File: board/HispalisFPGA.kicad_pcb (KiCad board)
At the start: 4 copper layers, 91.3 x 79.9 mm, 133 parts, among them J1 HC-TYPE-C-16P-01A, Q1 DMG1012T, Q2 DMG1012T, Q3 DMG1012T, Q4 DMG1012T, SW1 SW_DIP_x08, U1 93LC46B, U2 FT2232HQ, Y1 12MHz

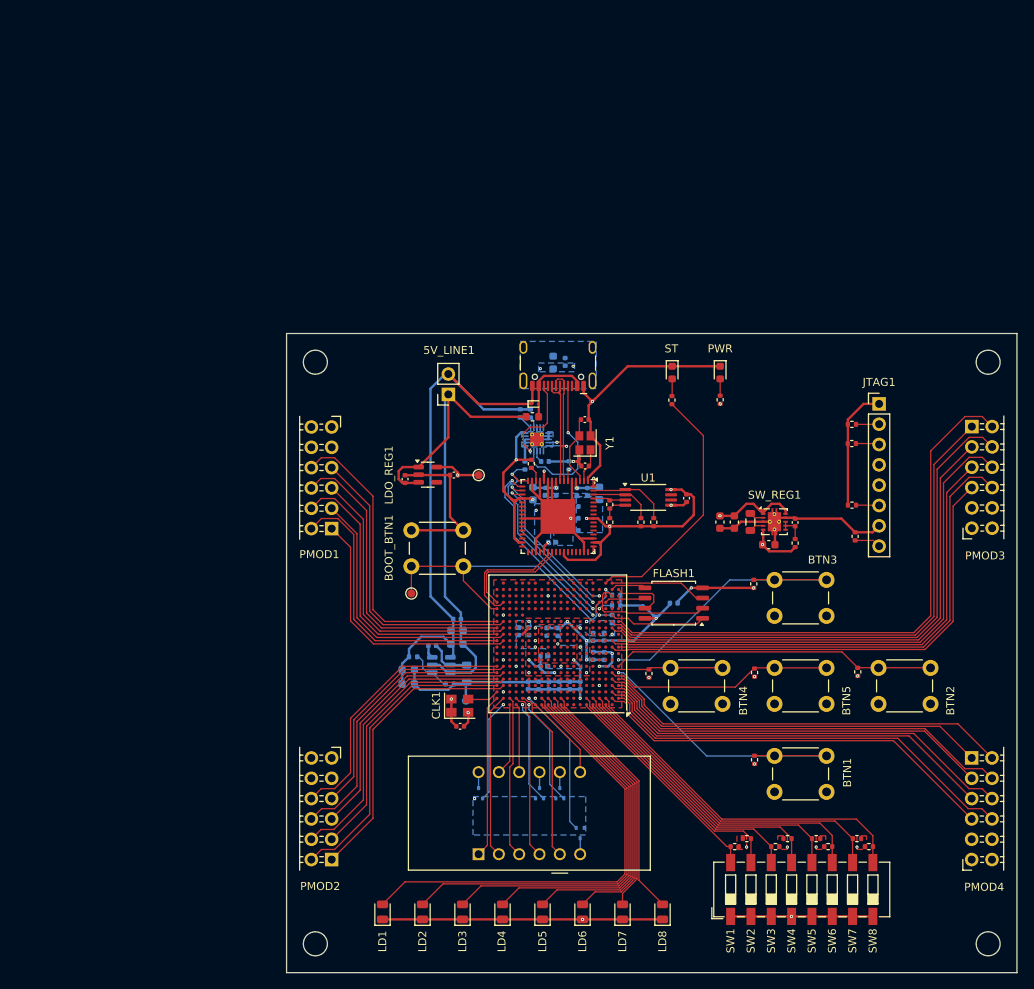
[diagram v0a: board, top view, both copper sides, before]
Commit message: Add metadata
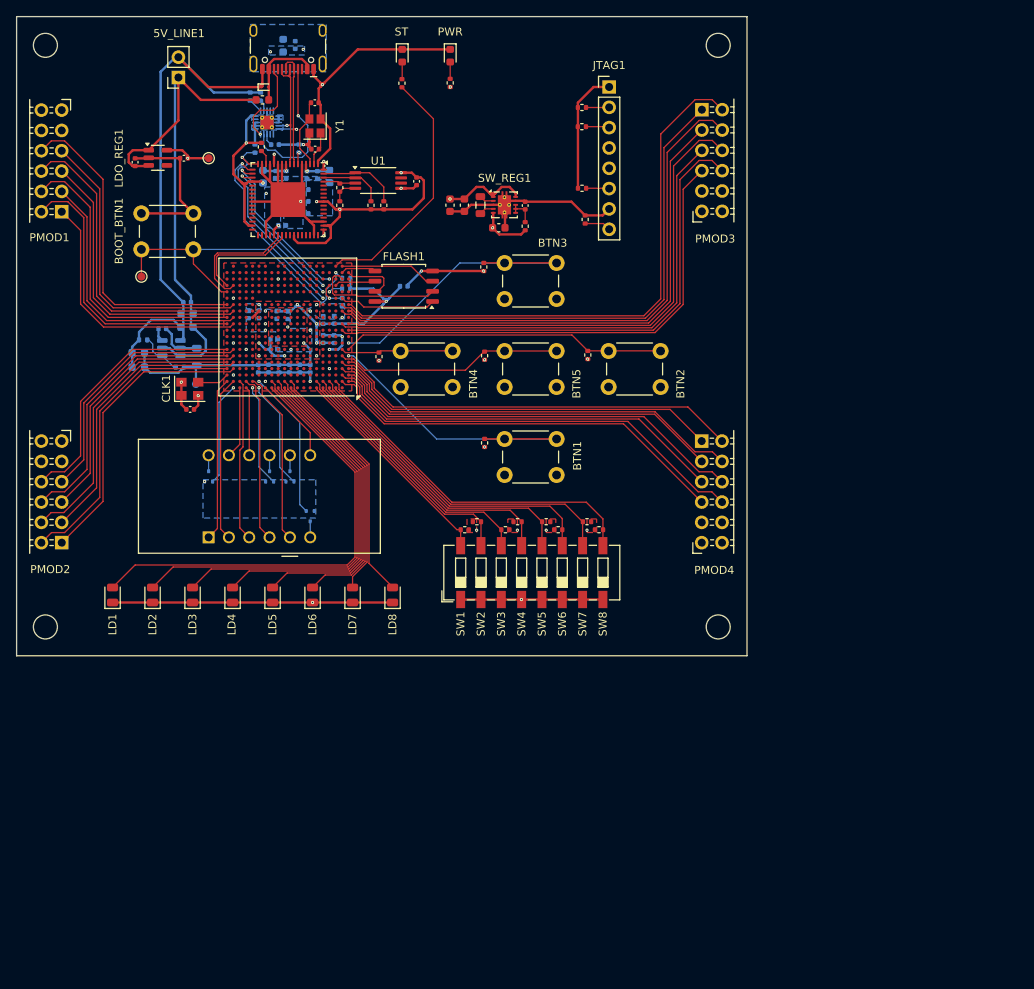
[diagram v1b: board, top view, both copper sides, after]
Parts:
- moved BTN2 52.0 mm to (102.6, 105.6)
- moved C37 52.0 mm to (66.9, 101.7)
- moved C45 52.0 mm to (77.0, 97.5)
- moved DISPLAY1 52.0 mm to (62.7, 128.9)
- moved FLASH1 52.0 mm to (77.0, 97.5)
- moved FPGA1 52.0 mm to (62.5, 102.6)
- moved LD1 52.0 mm to (40.6, 136.1)
- moved LD2 52.0 mm to (45.6, 136.1)
- moved LD3 52.0 mm to (50.6, 136.1)
- moved LD4 52.0 mm to (55.6, 136.1)
- moved LD5 52.0 mm to (60.6, 136.1)
- moved LD6 52.0 mm to (65.6, 136.1)
- moved LD7 52.0 mm to (70.6, 136.1)
- moved LD8 52.0 mm to (75.6, 136.1)
- moved R1 52.0 mm to (92.1, 90.0)
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
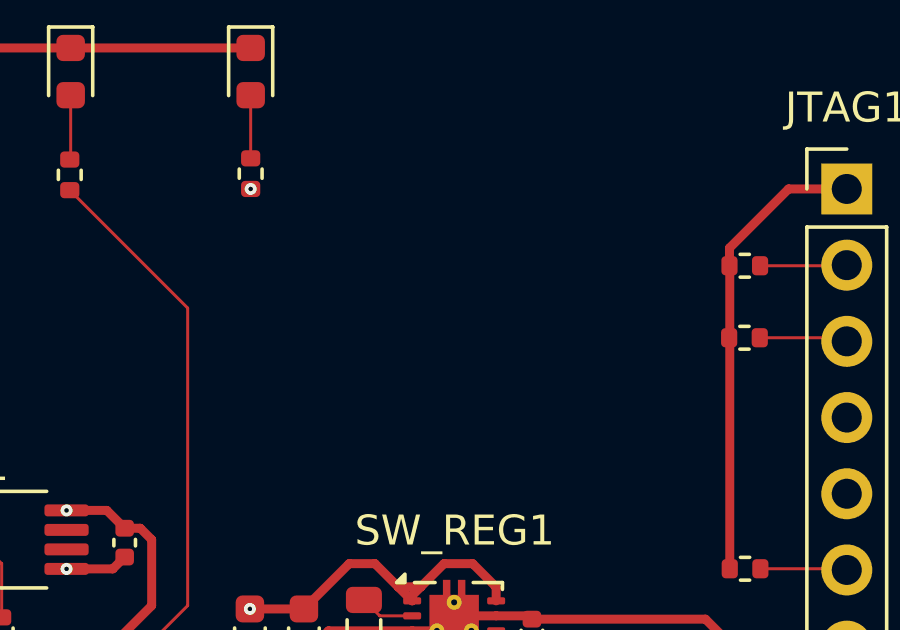
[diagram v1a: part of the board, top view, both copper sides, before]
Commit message: Add logo
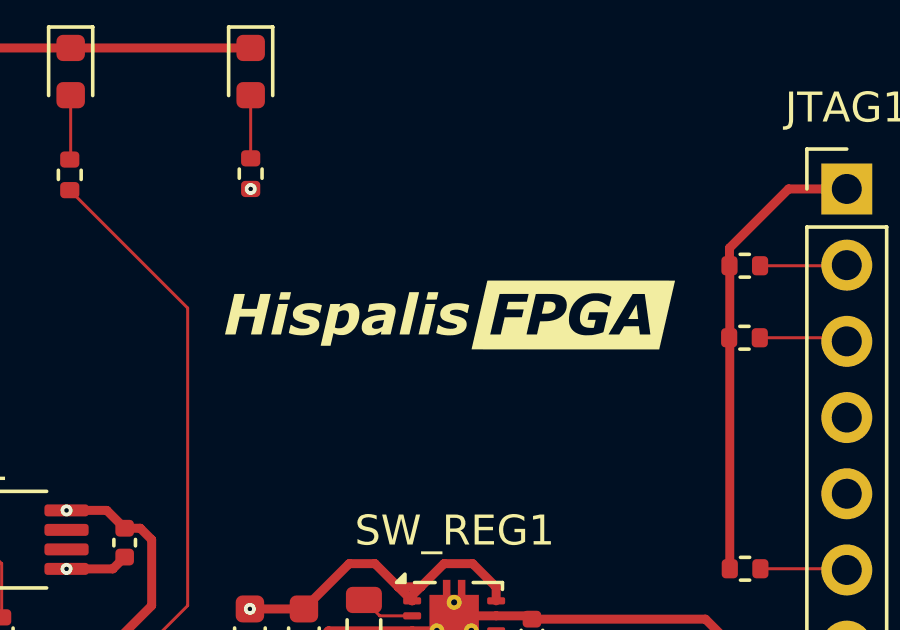
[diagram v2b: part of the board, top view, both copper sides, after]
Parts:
- added LOGO1: LOGO, HispalisFPGA:logo, F.Cu at (89.4, 76.8)
